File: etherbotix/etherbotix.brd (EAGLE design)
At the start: 100 x 50 mm, 107 parts, among them J1 J3011G21DNL, J2 22-03-5035, J3 22-03-5035, J4 22-03-5045, J5 22-03-5045, J6 1760510000, J7 1760490000, J8 502443-0470, J9 502443-0470, T1 TESTPAD, T2 TESTPAD, T3 TESTPAD, T4 TESTPAD, T5 TESTPAD, T6 TESTPAD, U1 STM32F407V, U2 TLK110, U3 OKI-78SR-5, U4 TLV1117, U5 ACS711ELCTR-25AB-T, U6 ACS711ELCTR-25AB-T, U7 MAX481CSA, U8 74LS126D, X1 25MHZ

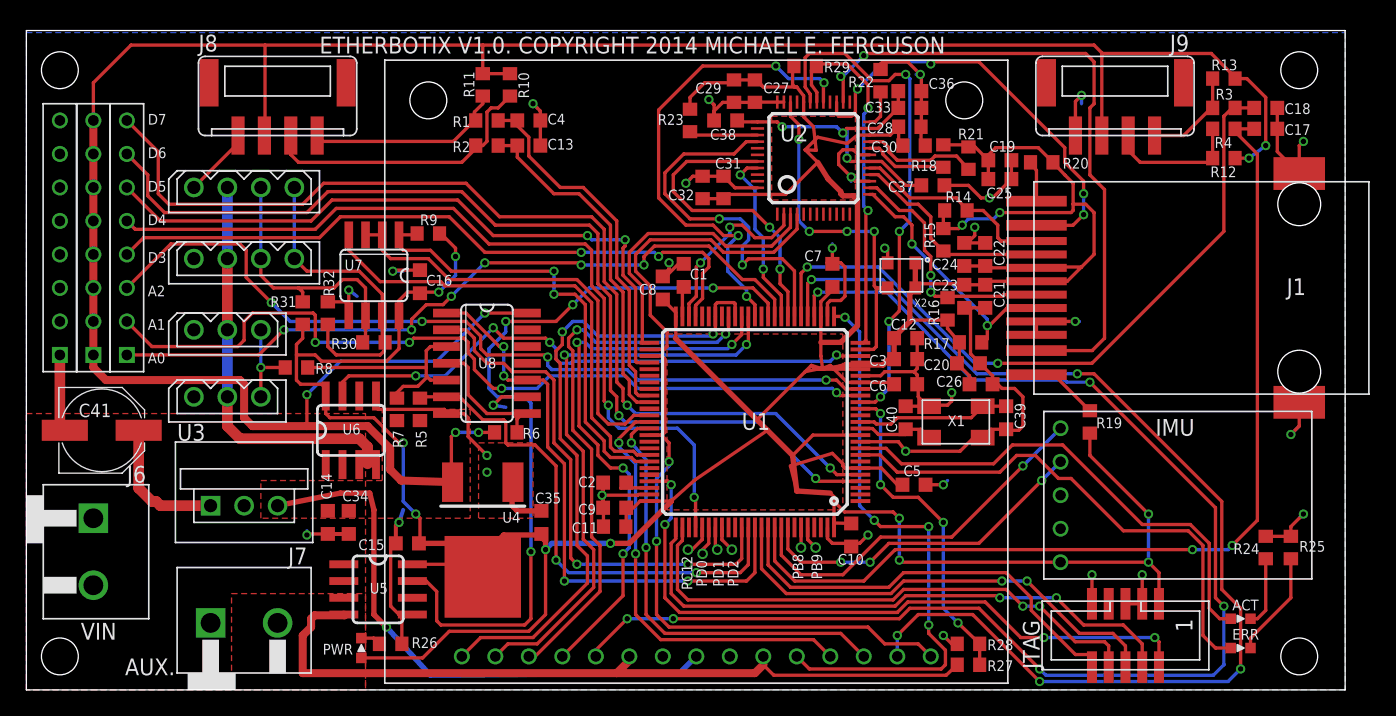
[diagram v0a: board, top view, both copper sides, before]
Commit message: some more refinements
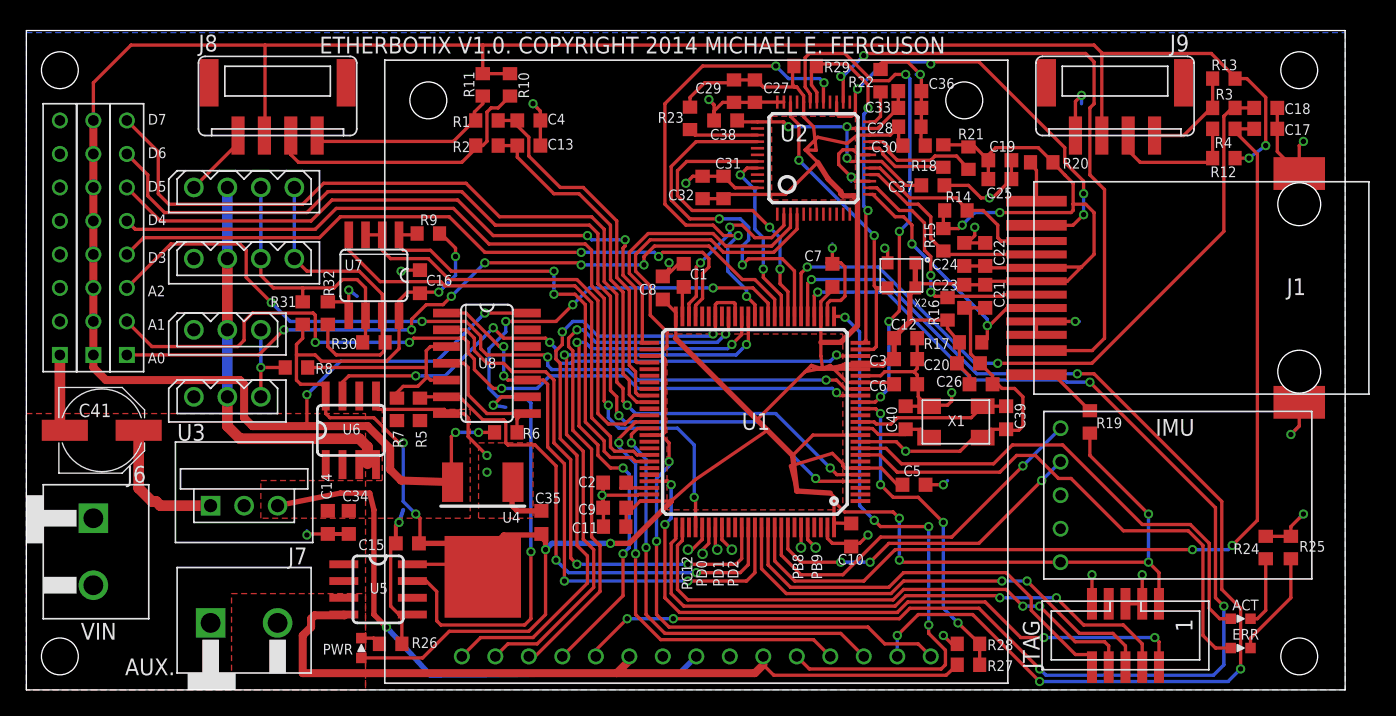
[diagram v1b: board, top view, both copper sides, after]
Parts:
- moved R23 0.16 mm to (50.3, 43.3)
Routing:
- net ETH_CLK: track 27.1 -> 24.2 mm, vias 4 -> 2
- net GND: track 204.1 -> 202.8 mm
- net N$24: track 23.9 -> 23.3 mm
